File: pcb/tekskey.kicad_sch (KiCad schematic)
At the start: 135 parts, among them J1 Conn_01x08, J2 Conn_01x08, SW0 MX_SW_HS, SW1 MX_SW_HS, SW10 MX_SW_HS, SW11 MX_SW_HS, SW12 MX_SW_HS, SW13 MX_SW_HS, SW14 MX_SW_HS, SW15 MX_SW_HS, SW1B1 MX_SW_HS, SW2 MX_SW_HS, SW20 MX_SW_HS, SW21 MX_SW_HS, SW22 MX_SW_HS, SW23 MX_SW_HS, SW24 MX_SW_HS, SW25 MX_SW_HS, SW2B1 MX_SW_HS, SW3 MX_SW_HS, SW30 MX_SW_HS, SW31 MX_SW_HS, SW32 MX_SW_HS, SW33 MX_SW_HS, SW34 MX_SW_HS, SW35 MX_SW_HS, SW3B1 MX_SW_HS, SW4 MX_SW_HS, SW40 MX_SW_HS, SW41 MX_SW_HS, SW42 MX_SW_HS, SW43 MX_SW_HS, SW44 MX_SW_HS, SW45 MX_SW_HS, SW4B1 MX_SW_HS, SW5 MX_SW_HS, SW50 MX_SW_HS, SW51 MX_SW_HS, SW51B1 MX_SW_HS, SW52 MX_SW_HS, SW53 MX_SW_HS, SW54 MX_SW_HS, SW55 MX_SW_HS, SW55B1 MX_SW_HS, SW5B1 MX_SW_HS

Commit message: cleanup routing
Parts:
- removed JP1, JP10, JP11, JP2, JP3, JP4, JP5, JP6, JP7, JP8, JP9: Jumper_2_Open, Jumper:SolderJumper-2_P1.3mm_Open_Pad1.0x1.5mm, symbol Jumper:Jumper_2_Open
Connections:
- net +5V: now also J1.7 (Pin_7)
- net GND: now also J1.8 (Pin_8)
- net LEDIN: now also J2.7 (Pin_7)
- net row5: now also SW51B1.1, SW55B1.1; no longer SW51B1.2, SW55B1.2
- net at D30.2 (A), SW55.1: now also SW55B1.2; no longer SW55B1.1
- net at LED51.2 (DOUT), LED52.3 (DIN): no longer LED6.2 (DOUT)
- net at LED51.3 (DIN): now also LED6.2 (DOUT); no longer LED50.2 (DOUT)
- net at D26.2 (A), SW51.1: now also SW51B1.2; no longer SW51B1.1
- net at LED40.2 (DOUT), LED50.3 (DIN): no longer LED6.3 (DIN)
- net at LED53.2 (DOUT), LED54.3 (DIN): no longer LED7.3 (DIN)
- net at LED55.3 (DIN): now also LED7.2 (DOUT); no longer LED54.2 (DOUT)
- net LEDOUT: no longer names the net of LED55.2 (DOUT)
- net LEDOUT: no longer LED7.2 (DOUT)
- new net: LED50.2 (DOUT), LED6.3 (DIN)
- new net: LED54.2 (DOUT), LED7.3 (DIN)
- no-connect marks 0 -> 2
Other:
- note removed: "LED Matrix"
- moved on the sheet: LED6, LED7, SW50, SW51, SW51B1, SW52, SW53, SW54, SW55, SW55B1

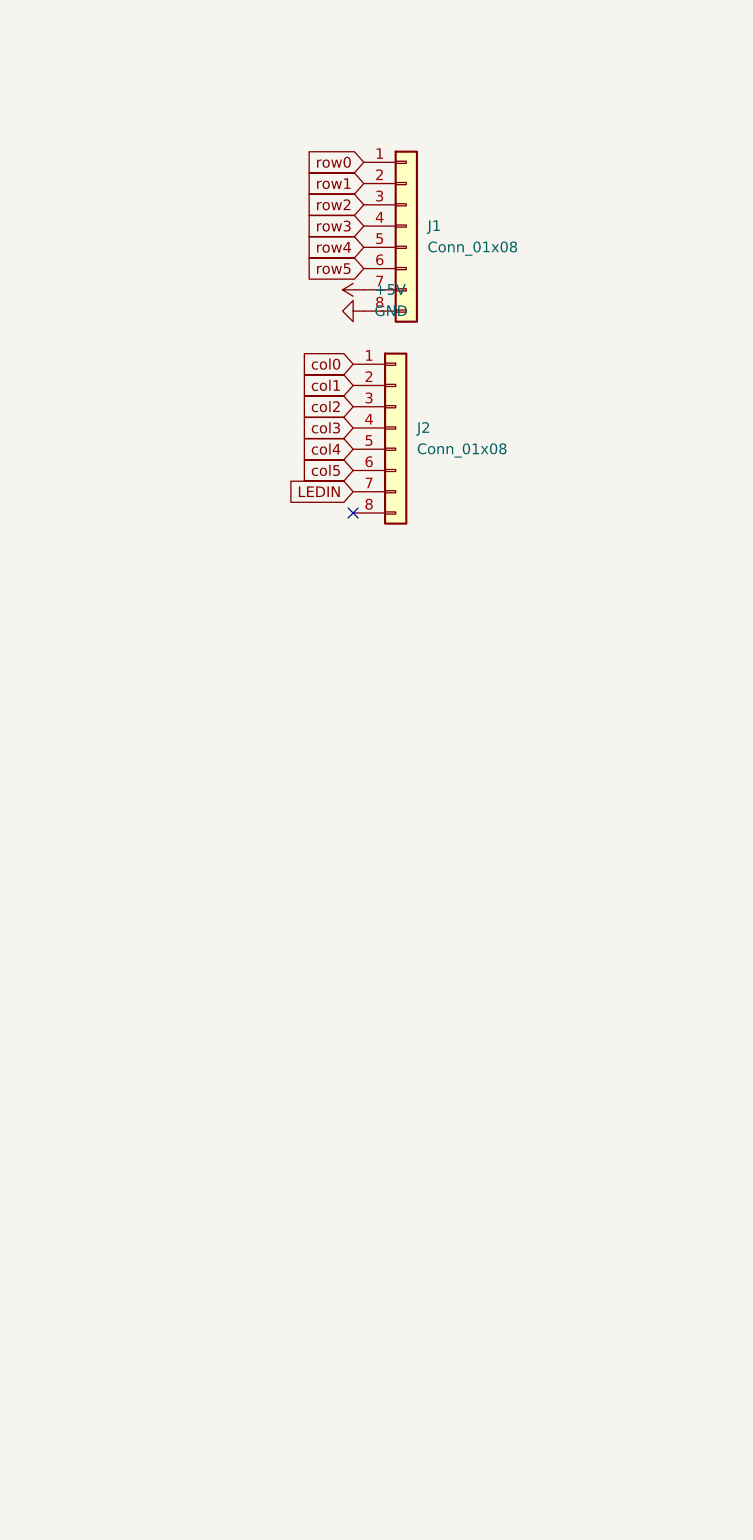
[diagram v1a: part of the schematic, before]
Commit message: wip
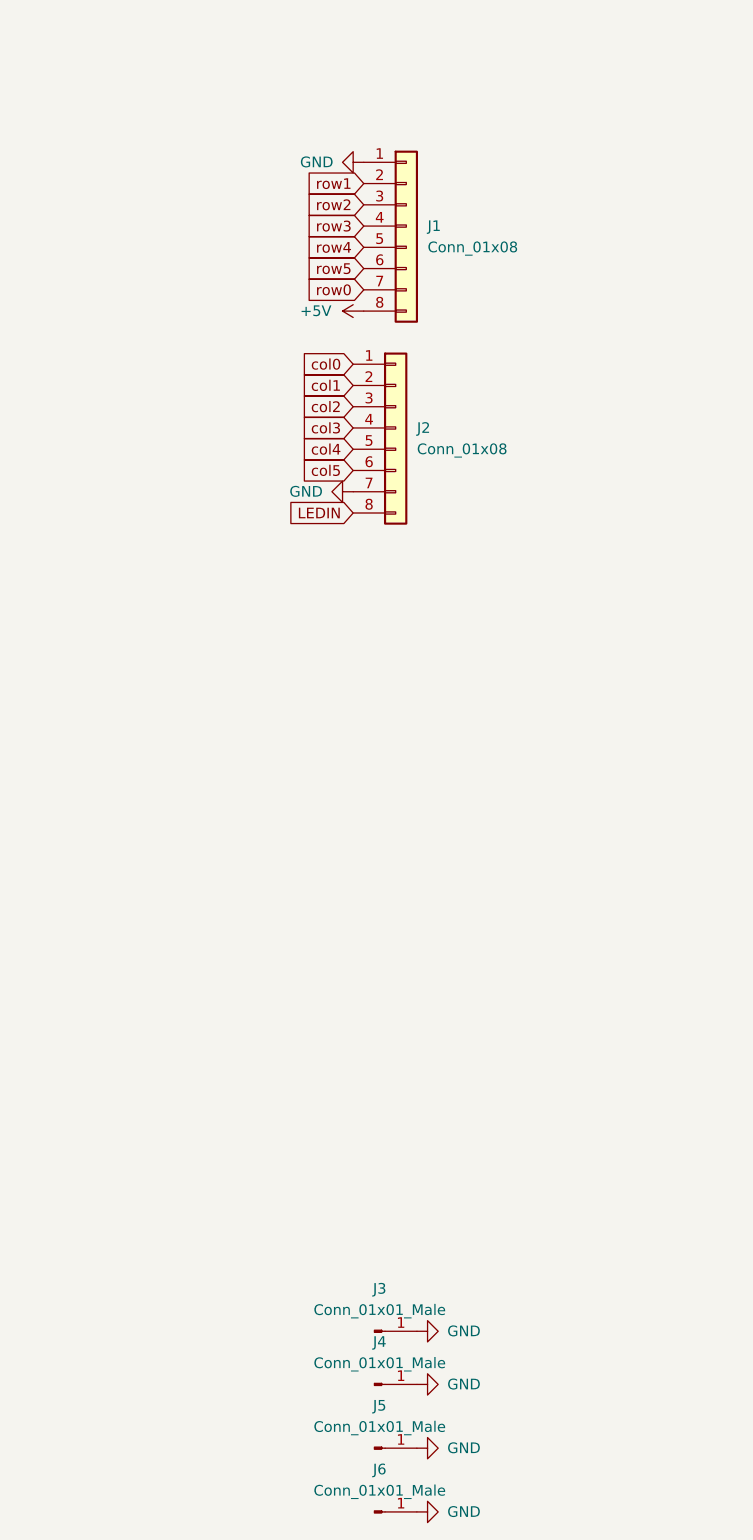
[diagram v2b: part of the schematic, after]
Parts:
- added J3, J4, J5, J6: Conn_01x01_Male, MountingHole:MountingHole_3.2mm_M3_DIN965_Pad, symbol Connector:Conn_01x01_Male
- D1, D10, D11, D12, D13, D14, D15, D16, D17, D18, D19, D2, D20, D21, D22, D23, D24, D25, D26, D27, D28, D29, D3, D30, D31, D32, D33, D34, D35, D36, D4, D5, D6, D7, D8, D9: footprint Diode_THT:D_DO-35_SOD27_P7.62mm_Horizontal -> custom:D_DO-35_SOD27_P7.62mm_Horizontal_NoSilk
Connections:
- net +5V: now also J1.8 (Pin_8); no longer J1.7 (Pin_7)
- net GND: now also J1.1 (Pin_1), J2.7 (Pin_7), J3.1 (Pin_1), J4.1 (Pin_1), J5.1 (Pin_1), J6.1 (Pin_1); no longer J1.8 (Pin_8)
- net LEDIN: now also J2.8 (Pin_8); no longer J2.7 (Pin_7)
- net row0: now also J1.7 (Pin_7); no longer J1.1 (Pin_1)
- no-connect marks 2 -> 1
